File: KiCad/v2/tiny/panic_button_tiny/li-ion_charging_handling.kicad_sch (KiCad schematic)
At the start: 7 parts, among them Q1 Si2301CDS, Q2 Si2305CDS, SW4 SPDT_Slide_SMD_6.7x2.6mm, U6 TP4056-42-ESOP8, U7 DW01A, U8 8205A

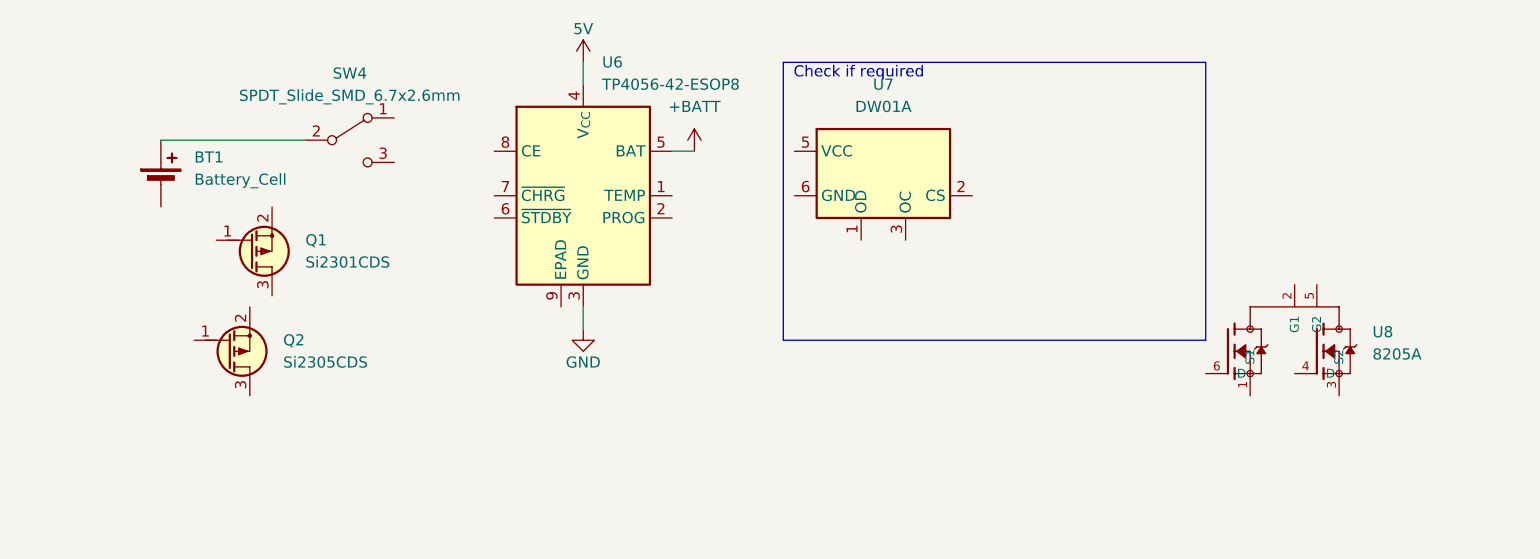
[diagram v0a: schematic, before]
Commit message: [UPDATE] connections in the circuits
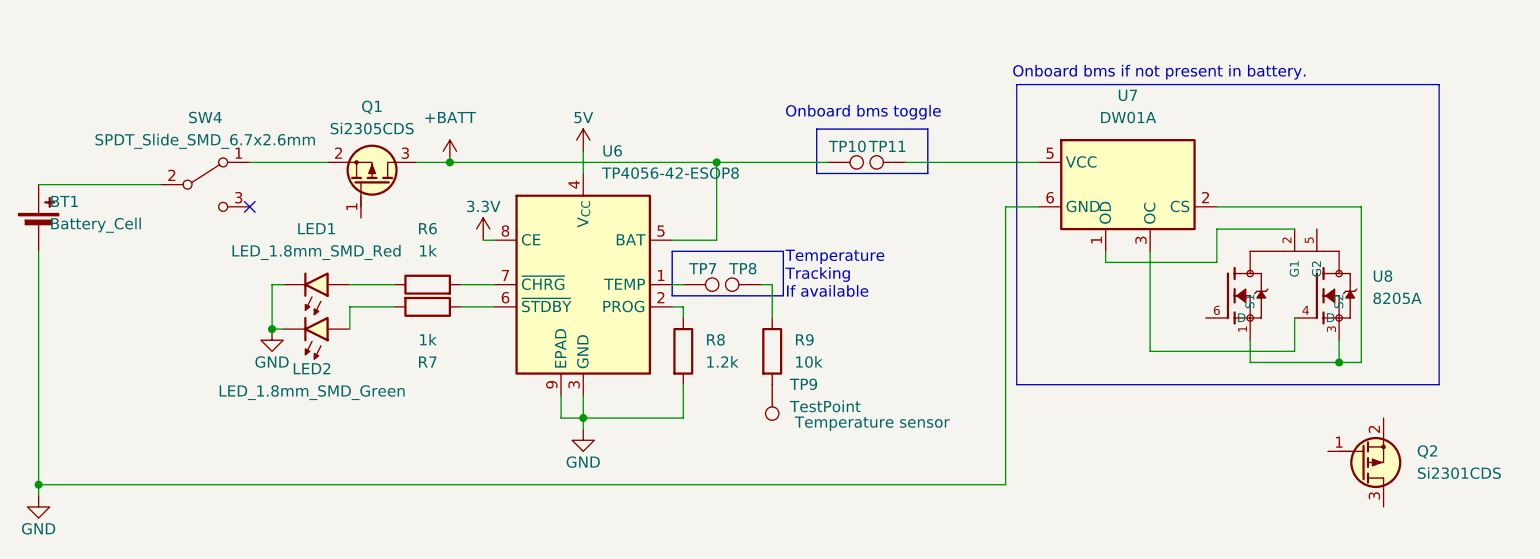
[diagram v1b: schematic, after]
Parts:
- added LED1: LED_1.8mm_SMD_Red, PCM_LED_SMD_AKL:LED_1.8mm_GullWing, symbol PCM_LED_AKL:LED_1.8mm_SMD_Red
- added LED2: LED_1.8mm_SMD_Green, PCM_LED_SMD_AKL:LED_1.8mm_GullWing, symbol PCM_LED_AKL:LED_1.8mm_SMD_Green
- added R6, R7: 1k_0603, PCM_Resistor_SMD_AKL:R_0603_1608Metric_Pad0.98x0.95mm_HandSolder, symbol PCM_4ms_Resistor:1k_0603
- added R8: 1.2k_0603, PCM_Resistor_SMD_AKL:R_0201_0603Metric_Pad0.64x0.40mm_HandSolder, symbol PCM_4ms_Resistor:1.2k_0603
- added R9: 10k_0603, PCM_Resistor_SMD_AKL:R_0603_1608Metric_Pad0.98x0.95mm_HandSolder, symbol PCM_4ms_Resistor:10k_0603
- added TP10, TP11, TP7, TP8: 1.25mm, TestPoint:TestPoint_2Pads_Pitch2.54mm_Drill0.8mm, symbol PCM_SparkFun-Connector:TestPoint_1.25mm
- added TP9: TestPoint, TestPoint:TestPoint_THTPad_D4.0mm_Drill2.0mm, symbol Connector:TestPoint
- renumbered Q2 to Q1, Q1 to Q2
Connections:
- net +BATT: now also Q1.3 (D), TP10.1
- net GND: now also BT1.2 (-), U6.9 (EPAD), U7.6 (GND), LED1.1 (K), LED2.1 (K), R8.2
- net at U7.1 (OD): now also U8.2 (G1)
- net at U7.2 (CS): now also U8.1 (S1), U8.3 (S2)
- net at U7.3 (OC): now also U8.4 (D)
- net at U7.5 (VCC): now also TP11.1
- net at SW4.1 (A): now also Q1.2 (S)
- net at U6.1 (TEMP): now also TP7.1
- net at U6.2 (PROG): now also R8.1
- net at U6.6 (~{STDBY}): now also R7.1
- net at U6.7 (~{CHRG}): now also R6.2
- net 3.3V: now reaches U6.8 (CE)
- new net: R9.2, TP9.1
- new net: LED2.2 (A), R7.2
- new net: LED1.2 (A), R6.1
- new net: R9.1, TP8.1
- no-connect marks 0 -> 1
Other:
- note added: "Onboard bms if not present in battery."
- note added: "Onboard bms toggle"
- note added: "Temperature Tracking If available"
- note removed: "Check if required"
- moved on the sheet: BT1, Q1, Q2, SW4, U6, U7, U8
